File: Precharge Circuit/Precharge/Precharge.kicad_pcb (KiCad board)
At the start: 2 copper layers, 2 parts

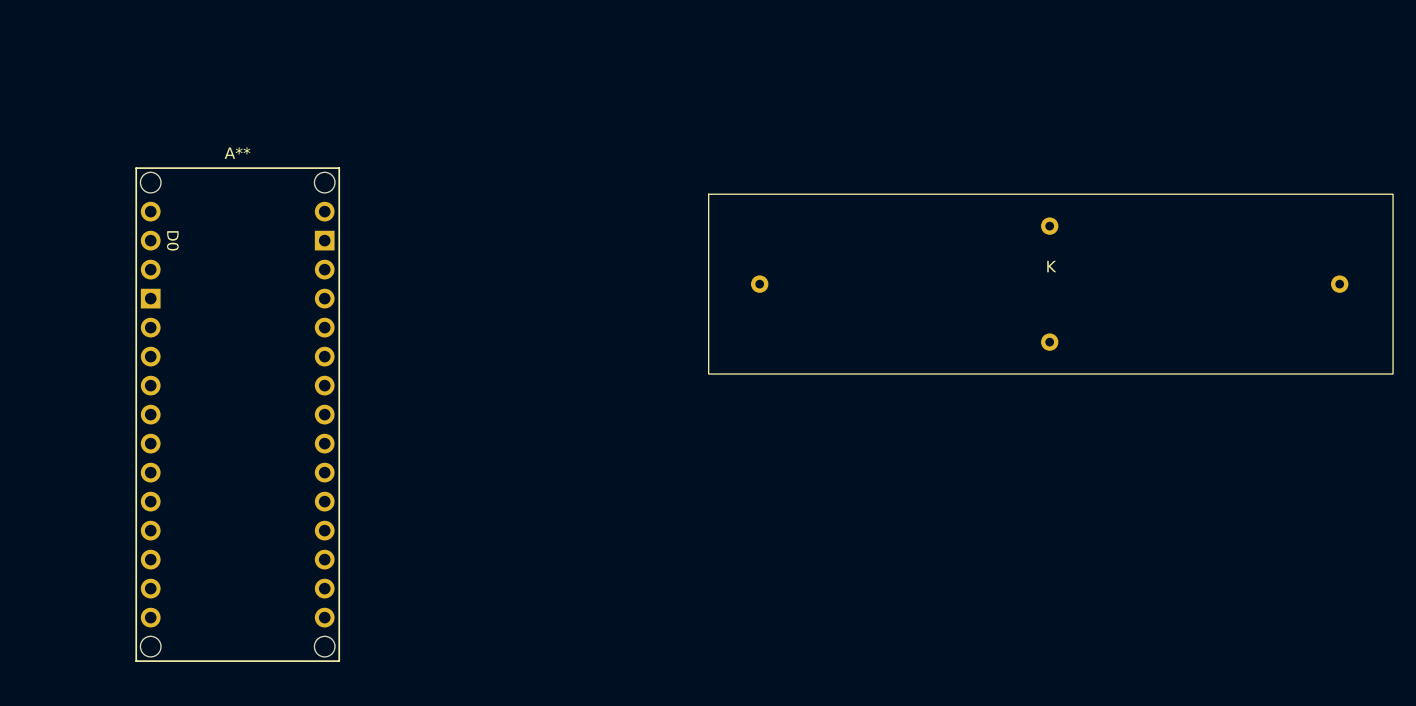
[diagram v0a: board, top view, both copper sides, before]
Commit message: Update
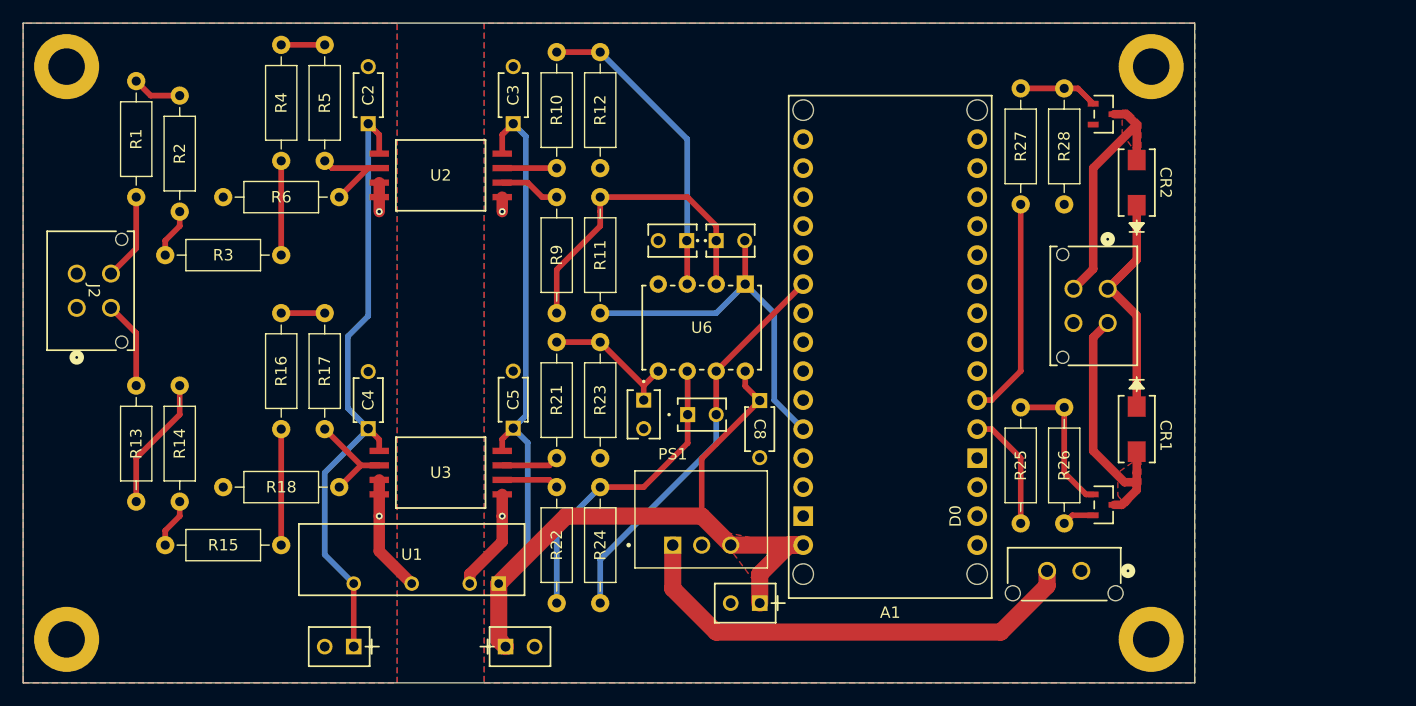
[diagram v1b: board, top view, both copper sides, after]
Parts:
- removed A**: Arduino_Nano_ESP32_Socket, PCM_arduino-library:Arduino_Nano_ESP32_Socket
- removed K: PreDisRelay, PrechargeRelays:PreDisRelay
- added A1: Arduino_Nano_33_IoT_Socket, PCM_arduino-library:Arduino_Nano_33_IoT_Socket, F.Cu at (181.6, 67.3)
- added C1: C324C106K3R5TA, 10uF Cap:CAP_C324C_MR_X7R_KEM, F.Cu at (170.2, 111.8)
- added C10: K331K15X7RF5TL2, 330pFCap:CAP_K-SERIES_15-L2_VIS, F.Cu at (160.0, 94.0)
- added C11: C324C106K3R5TA, 10uF Cap:CAP_C324C_MR_X7R_KEM, F.Cu at (134.6, 115.6)
- added C12: C324C106K3R5TA, 10uF Cap:CAP_C324C_MR_X7R_KEM, F.Cu at (147.9, 115.6)
- added C2: K104K10X7RF5UH5, 1uFCap:K104K10X7RF5UH5_VIS, F.Cu at (135.9, 69.8)
- added C3: K104K10X7RF5UH5, 1uFCap:K104K10X7RF5UH5_VIS, F.Cu at (148.6, 69.8)
- added C4: K104K10X7RF5UH5, 1uFCap:K104K10X7RF5UH5_VIS, F.Cu at (135.9, 96.5)
- added C5: K104K10X7RF5UH5, 1uFCap:K104K10X7RF5UH5_VIS, F.Cu at (148.6, 96.4)
- added C6: K331K15X7RF5TL2, 330pFCap:CAP_K-SERIES_15-L2_VIS, F.Cu at (163.8, 80.0)
- added C7: K331K15X7RF5TL2, 330pFCap:CAP_K-SERIES_15-L2_VIS, F.Cu at (166.4, 80.0)
- added C8: K104K10X7RF5UH5, 1uFCap:K104K10X7RF5UH5_VIS, F.Cu at (170.2, 94.0)
- added C9: K331K15X7RF5TL2, 330pFCap:CAP_K-SERIES_15-L2_VIS, F.Cu at (163.9, 95.2)
- added CR1: B240A-13-F, PreChargeParts:SMA_DIO-L, F.Cu at (203.2, 96.5)
- added CR2: B240A-13-F, PreChargeParts:SMA_DIO-L, F.Cu at (203.2, 74.9)
- added J1: 430450428, MolexVertical:CONN_SD-43045-010_04_MOL, F.Cu at (200.7, 84.2)
- added J2: 430450428, MolexVertical:CONN_SD-43045-010_04_MOL, F.Cu at (110.4, 85.9)
- added J4: 436500228, MolexVertical:CONN_SD-43650-010_02_MOL, F.Cu at (196.8, 109.2)
- added MOSFET1: DMN3404L-7, PreChargeParts:SOT23_DIO-L, F.Cu at (200.3, 103.2)
- added MOSFET2: DMN3404L-7, PreChargeParts:SOT23_DIO-L, F.Cu at (200.3, 68.9)
- added PS1: R-78E5.0-0.5, 12-5V Converter:CONV_R-78E5.0-0.5, F.Cu at (165.1, 104.4)
- added R1: 200k, Resistor_THT:R_Axial_DIN0207_L6.3mm_D2.5mm_P10.16mm_Horizontal, F.Cu at (115.6, 76.2)
- added R10: 1k, Resistor_THT:R_Axial_DIN0207_L6.3mm_D2.5mm_P10.16mm_Horizontal, F.Cu at (152.4, 73.7)
- added R11: 2.5k, Resistor_THT:R_Axial_DIN0207_L6.3mm_D2.5mm_P10.16mm_Horizontal, F.Cu at (156.2, 86.4)
- added R12: 2.5k, Resistor_THT:R_Axial_DIN0207_L6.3mm_D2.5mm_P10.16mm_Horizontal, F.Cu at (156.2, 73.7)
- added R13: 200k, Resistor_THT:R_Axial_DIN0207_L6.3mm_D2.5mm_P10.16mm_Horizontal, F.Cu at (115.6, 92.7)
- added R14: 200k, Resistor_THT:R_Axial_DIN0207_L6.3mm_D2.5mm_P10.16mm_Horizontal, F.Cu at (119.4, 92.7)
- added R15: 200k, Resistor_THT:R_Axial_DIN0207_L6.3mm_D2.5mm_P10.16mm_Horizontal, F.Cu at (118.1, 106.7)
- added R16: 200k, Resistor_THT:R_Axial_DIN0207_L6.3mm_D2.5mm_P10.16mm_Horizontal, F.Cu at (128.3, 96.5)
- added R17: 200k, Resistor_THT:R_Axial_DIN0207_L6.3mm_D2.5mm_P10.16mm_Horizontal, F.Cu at (132.1, 86.4)
- added R18: 10k, Resistor_THT:R_Axial_DIN0207_L6.3mm_D2.5mm_P10.16mm_Horizontal, F.Cu at (123.2, 101.6)
- added R2: 200k, Resistor_THT:R_Axial_DIN0207_L6.3mm_D2.5mm_P10.16mm_Horizontal, F.Cu at (119.4, 67.3)
- added R21: 1k, Resistor_THT:R_Axial_DIN0207_L6.3mm_D2.5mm_P10.16mm_Horizontal, F.Cu at (152.4, 99.1)
- added R22: 1k, Resistor_THT:R_Axial_DIN0207_L6.3mm_D2.5mm_P10.16mm_Horizontal, F.Cu at (152.4, 101.6)
- added R23: 2.5k, Resistor_THT:R_Axial_DIN0207_L6.3mm_D2.5mm_P10.16mm_Horizontal, F.Cu at (156.2, 99.1)
- added R24: 2.5k, Resistor_THT:R_Axial_DIN0207_L6.3mm_D2.5mm_P10.16mm_Horizontal, F.Cu at (156.2, 111.8)
- added R25: 200, Resistor_THT:R_Axial_DIN0207_L6.3mm_D2.5mm_P10.16mm_Horizontal, F.Cu at (193.0, 104.8)
- added R26: 10k, Resistor_THT:R_Axial_DIN0207_L6.3mm_D2.5mm_P10.16mm_Horizontal, F.Cu at (196.8, 94.6)
- added R27: 200, Resistor_THT:R_Axial_DIN0207_L6.3mm_D2.5mm_P10.16mm_Horizontal, F.Cu at (193.0, 76.8)
- added R28: 10k, Resistor_THT:R_Axial_DIN0207_L6.3mm_D2.5mm_P10.16mm_Horizontal, F.Cu at (196.8, 66.7)
- added R3: 200k, Resistor_THT:R_Axial_DIN0207_L6.3mm_D2.5mm_P10.16mm_Horizontal, F.Cu at (118.1, 81.3)
- added R4: 200k, Resistor_THT:R_Axial_DIN0207_L6.3mm_D2.5mm_P10.16mm_Horizontal, F.Cu at (128.3, 73.0)
- added R5: 200k, Resistor_THT:R_Axial_DIN0207_L6.3mm_D2.5mm_P10.16mm_Horizontal, F.Cu at (132.1, 62.9)
- added R6: 10k, Resistor_THT:R_Axial_DIN0207_L6.3mm_D2.5mm_P10.16mm_Horizontal, F.Cu at (123.2, 76.2)
- added R9: 1k, Resistor_THT:R_Axial_DIN0207_L6.3mm_D2.5mm_P10.16mm_Horizontal, F.Cu at (152.4, 76.2)
- added REF**: MountingHole_3.2mm_M3_ISO7380_Pad, MountingHole:MountingHole_3.2mm_M3_ISO7380_Pad, F.Cu at (204.5, 114.9)
- added REF**: MountingHole_3.2mm_M3_ISO7380_Pad, MountingHole:MountingHole_3.2mm_M3_ISO7380_Pad, F.Cu at (109.5, 64.8)
- added REF**: MountingHole_3.2mm_M3_ISO7380_Pad, MountingHole:MountingHole_3.2mm_M3_ISO7380_Pad, F.Cu at (204.5, 64.8)
- added REF**: MountingHole_3.2mm_M3_ISO7380_Pad, MountingHole:MountingHole_3.2mm_M3_ISO7380_Pad, F.Cu at (109.5, 114.9)
- added U1: TEA 1-0505E, PreChargeParts:TEA 1E_TRP, F.Cu at (147.3, 110.0)
- added U2: AMC1351DWVR, AMC 1351:SOIC8_DWV_TEX, F.Cu at (142.2, 74.3)
- added U3: AMC1351DWVR, AMC 1351:SOIC8_DWV_TEX, F.Cu at (142.2, 100.3)
- added U6: OP284EPZ, OP284:N_8_ADI, F.Cu at (168.9, 83.8)
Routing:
- net /+5: track 0.00 -> 106.9 mm
- net /HV+5: track 0.00 -> 55.3 mm
- net Net-(PS1-+VIN): track 0.00 -> 41.2 mm
- net Net-(U6-OUTB): track 0.00 -> 35.3 mm
- net Net-(U6-OUTA): track 0.00 -> 32.4 mm
- net Net-(U6--INA): track 0.00 -> 28.0 mm
- net Net-(U6--INB): track 0.00 -> 27.3 mm
- net Net-(U6-+INA): track 0.00 -> 27.3 mm
- net Net-(MOSFET1-D): track 0.00 -> 22.6 mm
- net Net-(MOSFET2-D): track 0.00 -> 22.1 mm
- net /ShutdownIn: track 0.00 -> 19.9 mm
- net Net-(A1-PadD3): track 0.00 -> 19.5 mm
- net GND: track 0.00 -> 13.4 mm, vias 0 -> 2
- net Net-(MOSFET1-G): track 0.00 -> 12.9 mm
- net /HVGND: track 0.00 -> 12.8 mm, vias 0 -> 2
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- added copper zone on F.Cu, net /+5
- added copper zone on B.Cu, net /HVGND
- added copper zone on F.Cu, net /HVGND
- added copper zone on B.Cu, net GND
- added copper zone on F.Cu, net GND
- added copper zone on F.Cu, net Net-(MOSFET1-D)
- added copper zone on F.Cu, net Net-(MOSFET2-D)
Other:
- board outline added: 102.6 x 57.8 mm
